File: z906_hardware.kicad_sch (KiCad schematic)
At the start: 32 parts, among them J1 USB_C_Receptacle_USB2.0_14P, J3 DE_15 Amplifier, J4 DE15 Console, U1 ESP32-S3-WROOM-1, U2 AP63203WU, U3 PCM5102A, U4 TPD2EUSB30, U5 TPD1E05U06DYA, U6 TPS7A4533, U7 PCM1860DBT

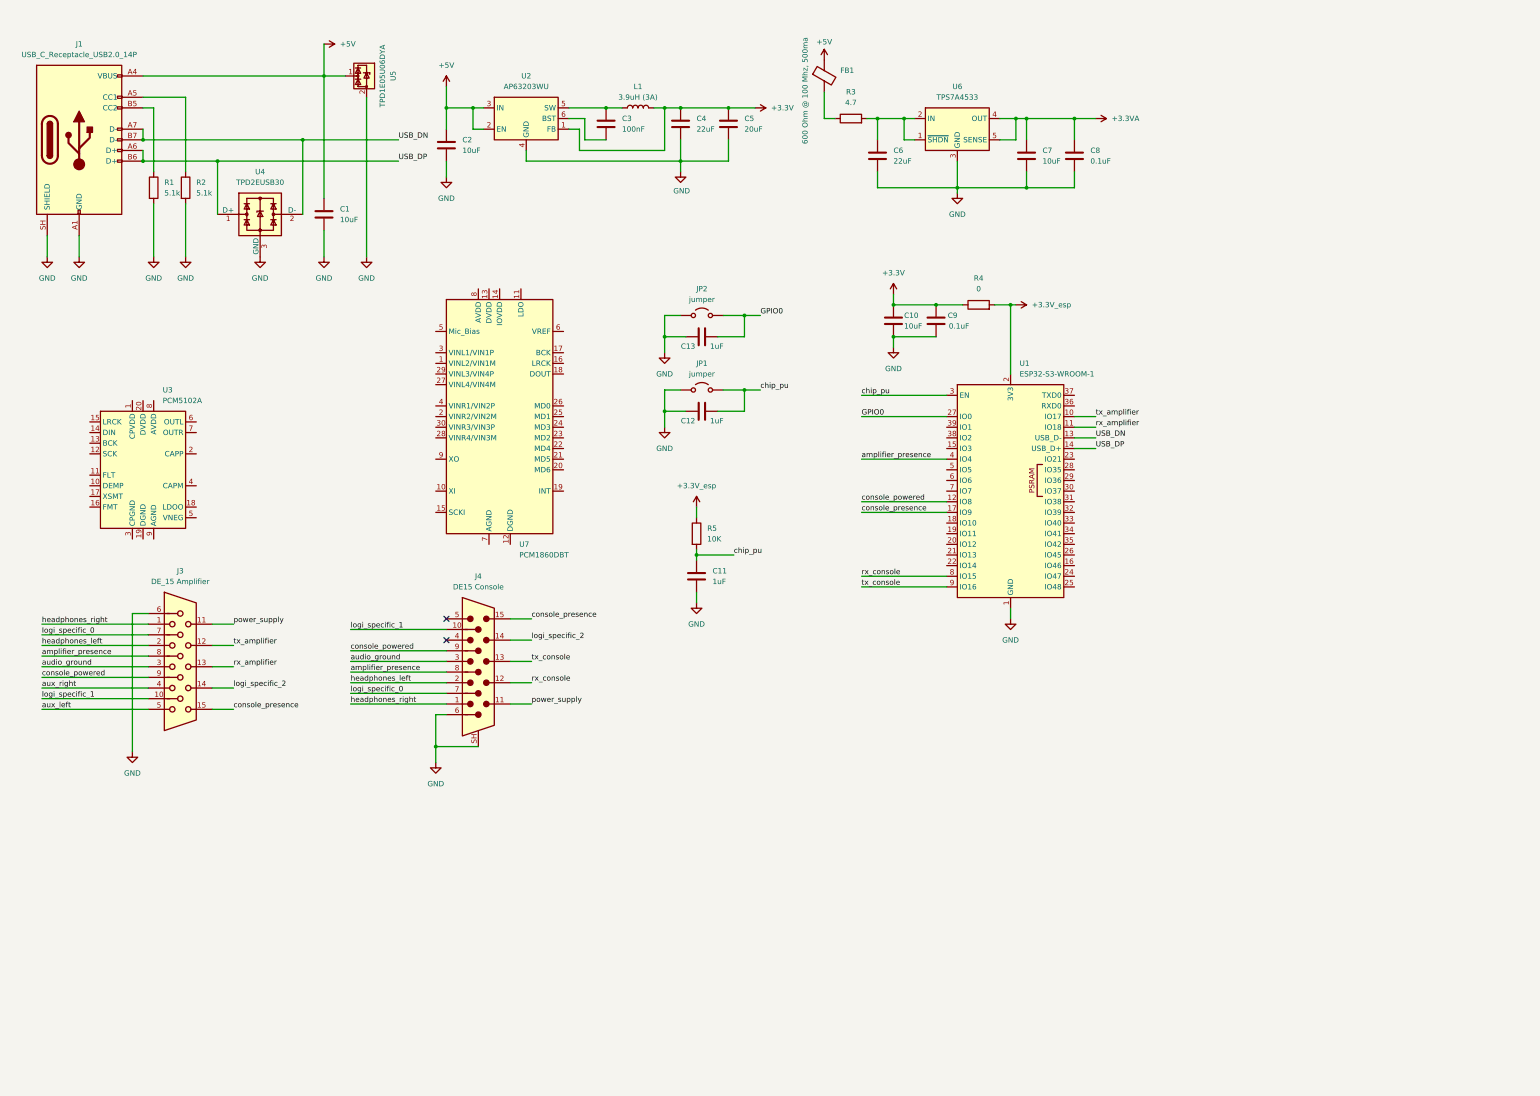
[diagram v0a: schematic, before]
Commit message: PCM5102A
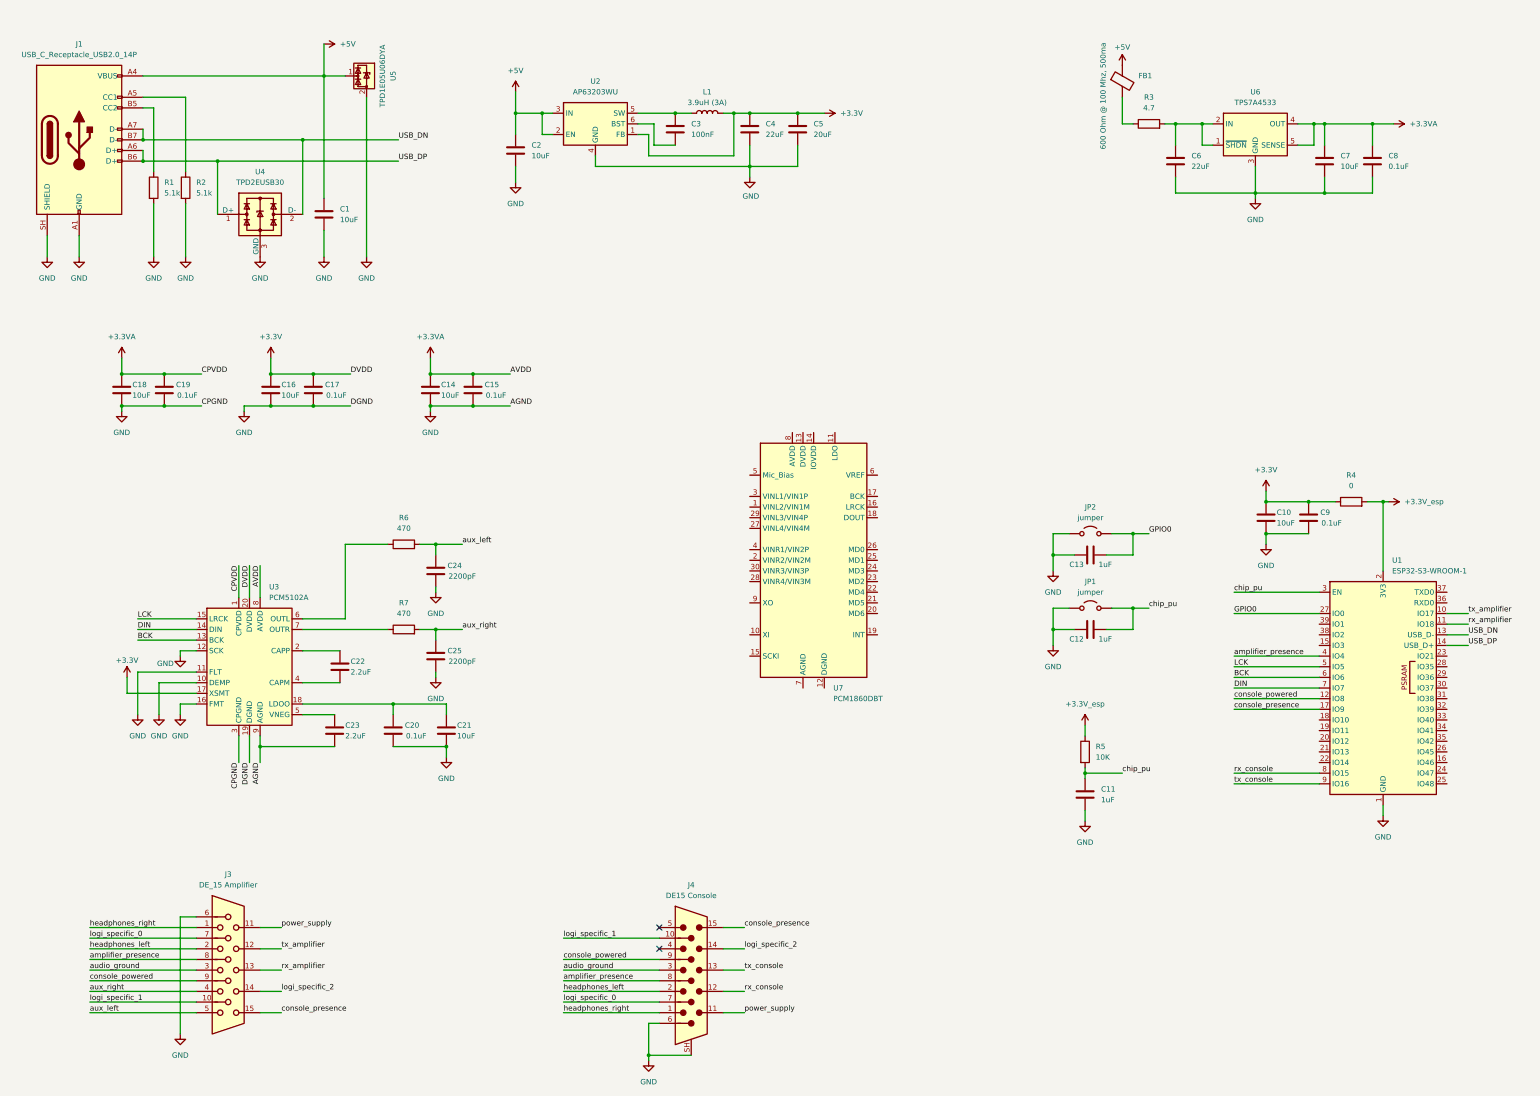
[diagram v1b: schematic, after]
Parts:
- added C14, C16, C18, C21: 10uF, symbol Device:C
- added C15, C17, C19, C20: 0.1uF, symbol Device:C
- added C22, C23: 2.2uF, symbol Device:C
- added C24, C25: 2200pF, symbol Device:C
- added R6, R7: 470, symbol Device:R
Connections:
- net +3.3V: now also U3.17 (XSMT), U3.20 (DVDD), C16.1, C17.1
- net +3.3VA: now also U3.1 (CPVDD), U3.8 (AVDD), C14.1, C15.1, C18.1, C19.1
- net GND: now also U3.10 (DEMP), U3.11 (FLT), U3.12 (SCK), U3.16 (FMT), U3.19 (DGND), U3.3 (CPGND), U3.9 (AGND), C14.2, C15.2, C16.2, C17.2, C18.2, C19.2, C20.2, C21.2, C23.2, C24.2, C25.2
- net aux_left: now also C24.1, R6.2
- net aux_right: now also C25.1, R7.2
- net LCK: now reaches U1.5 (IO5)
- net LCK: now also U3.15 (LRCK)
- net BCK: now reaches U1.6 (IO6)
- net BCK: now also U3.13 (BCK)
- net DIN: now reaches U1.7 (IO7)
- net DIN: now also U3.14 (DIN)
- net at U3.18 (LDOO): now also C20.1, C21.1
- net at U3.2 (CAPP): now also C22.1
- net at U3.4 (CAPM): now also C22.2
- net at U3.5 (VNEG): now also C23.1
- net at U3.6 (OUTL): now also R6.1
- net at U3.7 (OUTR): now also R7.1
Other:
- moved on the sheet: C10, C11, C12, C13, C2, C3, C4, C5, C6, C7, C8, C9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

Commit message: PCM1860DBT
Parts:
- added C26, C28, C30, C32: 10uF, symbol Device:C
- added C27, C29, C31, C33: 0.1uF, symbol Device:C
- added C34: 1uF, symbol Device:C
- added C35, C37: 4.7uF, symbol Device:C
- added C36, C38: 1nF, symbol Device:C
- added J2: AudioJack3, symbol Connector_Audio:AudioJack3
- added R10, R11: 100k, symbol Device:R
- added R12, R9: 100, symbol Device:R
- added R8: 10K, symbol Device:R
- added U8: TPD2E2U06DCK, Package_TO_SOT_SMD:SOT-323_SC-70, symbol Power_Protection:TPD2E2U06DCK
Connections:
- net +3.3V: now also U7.13 (DVDD), U7.14 (IOVDD), C26.1, C27.1, C28.1, C29.1, R8.1
- net +3.3VA: now also U7.8 (AVDD), C30.1, C31.1
- net BCK: now also U7.17 (BCK)
- net GND: now also U7.10 (XI), U7.12 (DGND), U7.20 (MD6), U7.21 (MD5), U7.22 (MD4), U7.23 (MD2), U7.24 (MD3), U7.25 (MD1), U7.26 (MD0), U7.7 (AGND), C26.2, C27.2, C28.2, C29.2, C30.2, C31.2, C32.2, C33.2, C34.2, C36.1, C38.1, J2.S, R10.1, R11.1, U8.3; no longer U3.12 (SCK)
- net LCK: now also U7.16 (LRCK)
- net at U7.11 (LDO): now also C32.1, C33.1
- net MCLK: now reaches U7.15 (SCKI)
- net MCLK: now also U1.19 (IO11), U3.12 (SCK)
- net ADC_DATA: now reaches U7.18 (DOUT)
- net ADC_DATA: now also U1.7 (IO7)
- net at U7.19 (INT): now also R8.2
- net at U7.3 (VINL1/VIN1P): now also C36.2, R9.2
- net at U7.4 (VINR1/VIN2P): now also C38.2, R12.2
- net at U7.6 (VREF): now also C34.1
- net DAC_DATA: now reaches U1.18 (IO10)
- net DAC_DATA: now also U3.14 (DIN)
- removed net DIN: U1.7 (IO7), U3.14 (DIN)
- new net: C35.1, J2.T, R10.2, U8.1
- new net: C37.1, J2.R, R11.2, U8.2
- new net: C37.2, R12.1
- new net: C35.2, R9.1
- no-connect marks 2 -> 9
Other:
- moved on the sheet: C10, C11, C12, C13, C14, C15, C16, C17, C18, C19, C20, C21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
